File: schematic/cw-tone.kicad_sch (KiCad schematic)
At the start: 21 parts, among them Q14 2N7000, Q15 2N7000, U16 NE5532

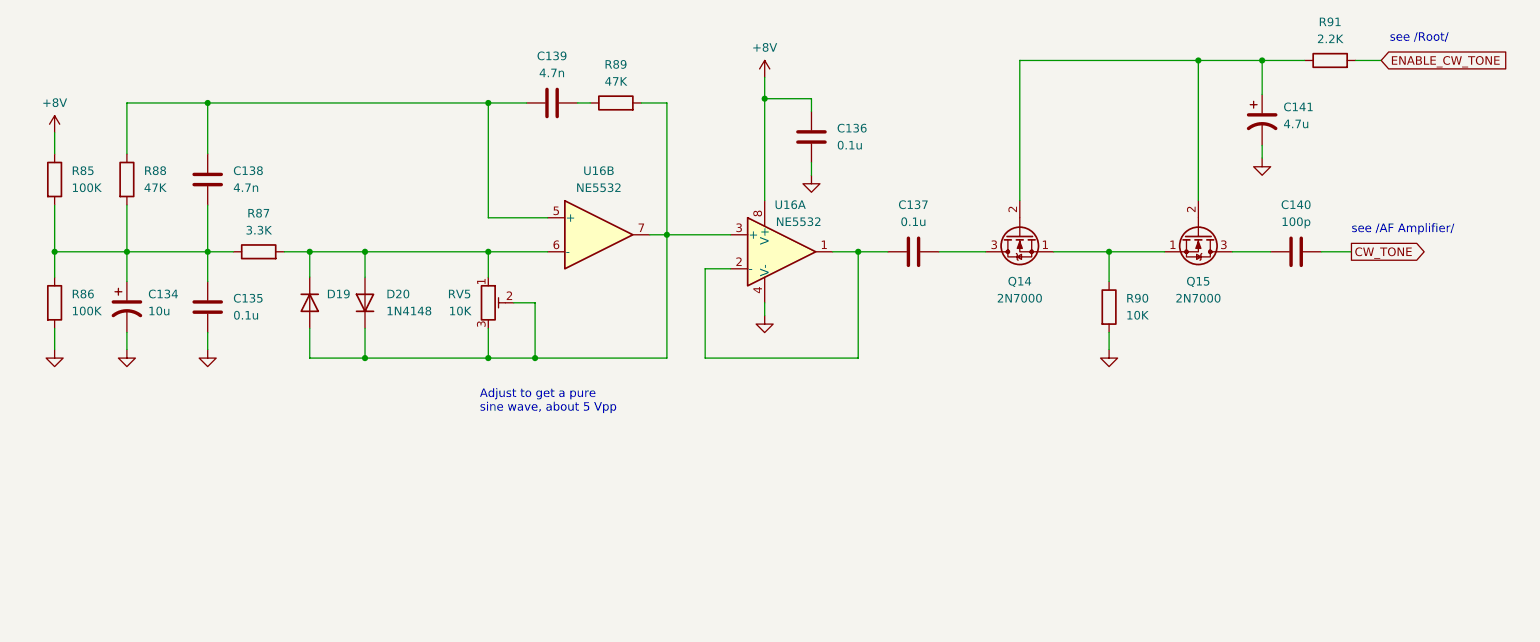
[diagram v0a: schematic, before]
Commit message: Minor changes
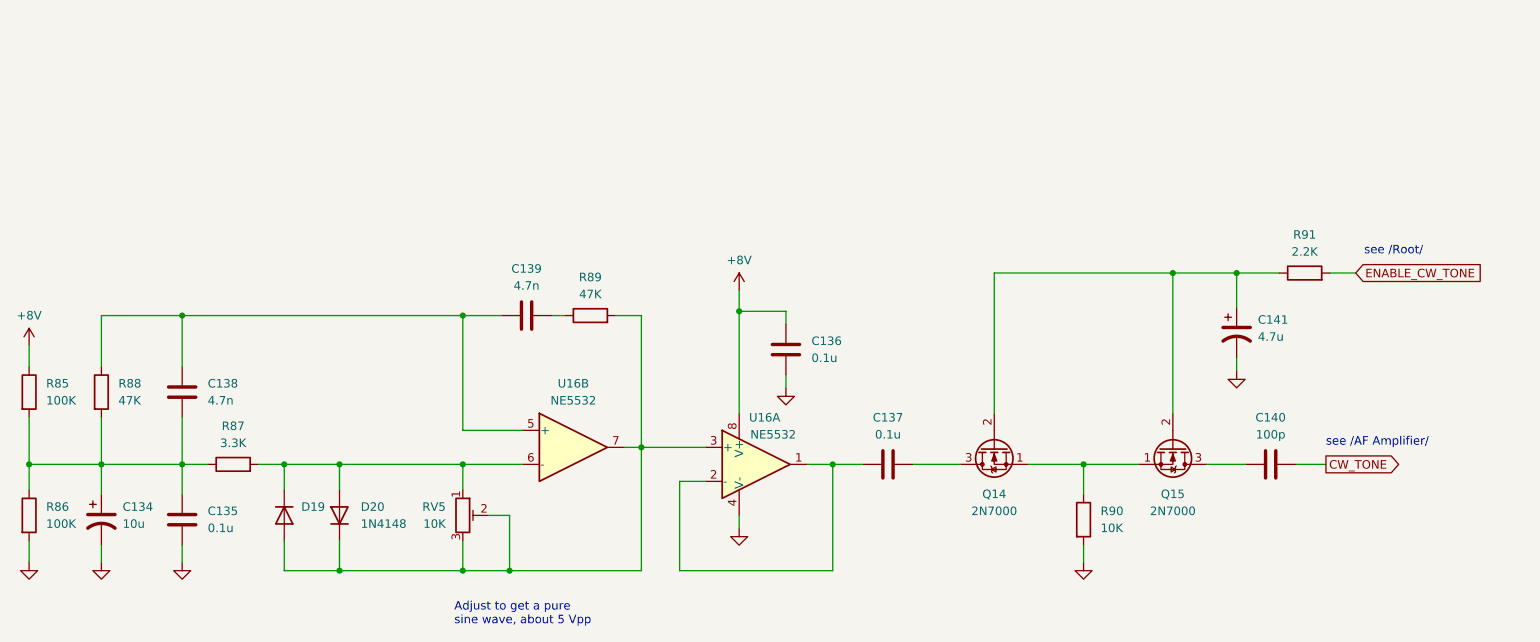
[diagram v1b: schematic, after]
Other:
- moved on the sheet: C134, C135, C136, C137, C138, C139, C140, C141, D19, D20, Q14, Q15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
